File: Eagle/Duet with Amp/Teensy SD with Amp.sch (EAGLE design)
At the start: 20 parts, among them IC2 LM386N-1

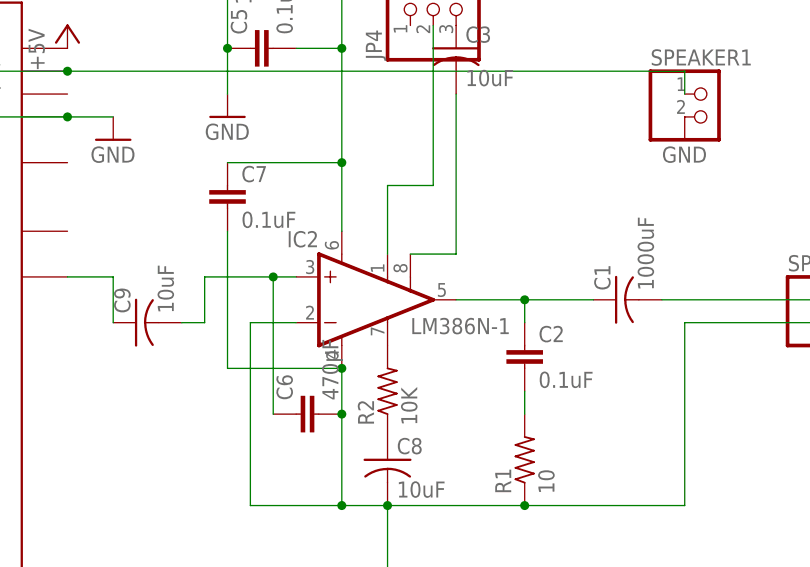
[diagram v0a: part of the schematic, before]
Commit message: Revert "Traced to 32mils"
This reverts commit ffbe95997752b5ed6823b856a1fed8613c21e4f0.
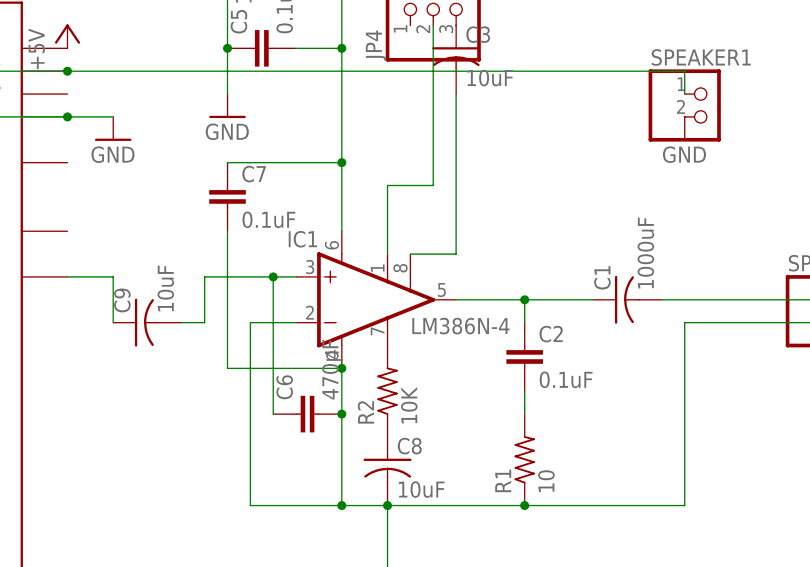
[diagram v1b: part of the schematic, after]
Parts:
- removed IC2: LM386N-1, linear:LM386N-1
- added IC1: LM386N-4, linear:LM386N-4
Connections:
- net +5V: now also IC1.VS; no longer IC2.VS
- net GND: now also IC1.-IN, IC1.GND; no longer IC2.-IN, IC2.GND
- net N$2: now also IC1.GAIN@2; no longer IC2.GAIN@2
- net N$26: now also IC1.GAIN@1; no longer IC2.GAIN@1
- net N$3: now also IC1.OUT; no longer IC2.OUT
- net N$4: now also IC1.BYPASS; no longer IC2.BYPASS
- net N$6: now also IC1.+IN; no longer IC2.+IN
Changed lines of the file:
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@@
 </classes>
 <parts>
+<part name="IC1" library="linear" deviceset="LM386?-*" device="N" technology="4"/>
 <part name="C3" library="rcl" deviceset="C-US" device="025-030X050" value="10uF"/>
 <part name="C8" library="rcl" deviceset="C-US" device="025-030X050" value="10uF"/>
-<part name="C7" library="capacitor-wima" library_urn="urn:adsk.eagle:library:116" deviceset="C" device="2.5/4" value="0.1uF"/>
+<part name="C7" library="capacitor-wima" deviceset="C" device="2.5/4" value="0.1uF"/>
 <part name="R1" library="resistor" deviceset="R-US_" device="0207/7" value="10"/>
 <part name="R2" library="resistor" deviceset="R-US_" device="0207/7" value="10K"/>
-<part name="C2" library="capacitor-wima" library_urn="urn:adsk.eagle:library:116" deviceset="C" device="2.5/4" value="0.1uF"/>
-<part name="C6" library="capacitor-wima" library_urn="urn:adsk.eagle:library:116" deviceset="C" device="2.5/4" value="470pF"/>
+<part name="C2" library="capacitor-wima" deviceset="C" device="2.5/4" value="0.1uF"/>
+<part name="C6" library="capacitor-wima" deviceset="C" device="2.5/4" value="470pF"/>
 <part name="C1" library="rcl" deviceset="C-US" device="025-030X050" value="1000uF"/>
 <part name="SPEAKER" library="pinhead" deviceset="PINHD-1X2" device=""/>
 <part name="C4" library="rcl" deviceset="C-US" device="025-030X050" value="100uF"/>
-<part name="C5" library="capacitor-wima" library_urn="urn:adsk.eagle:library:116" deviceset="C" device="2.5/4" value="0.1uF"/>
-<part name="P+3" library="supply1" library_urn="urn:adsk.eagle:library:371" deviceset="+5V" device=""/>
+<part name="C5" library="capacitor-wima" deviceset="C" device="2.5/4" value="0.1uF"/>
+<part name="P+3" library="supply1" deviceset="+5V" device=""/>
 <part name="U$1" library="Teensy_3_and_LC_Series_Boards_v1.4" deviceset="TEENSY_3.1-3.2_OUTER_ROW" device=""/>
-<part name="GND3" library="supply1" library_urn="urn:adsk.eagle:library:371" deviceset="GND" device=""/>
-<part name="P+1" library="supply1" library_urn="urn:adsk.eagle:library:371" deviceset="+5V" device=""/>
+<part name="GND3" library="supply1" deviceset="GND" device=""/>
+<part name="P+1" library="supply1" deviceset="+5V" device=""/>
 <part name="JP1" library="pinhead" deviceset="PINHD-1X7" device=""/>
 <part name="JP2" library="pinhead" deviceset="PINHD-1X4" device=""/>
-<part name="P+2" library="supply1" library_urn="urn:adsk.eagle:library:371" deviceset="+5V" device=""/>
-<part name="GND4" library="supply1" library_urn="urn:adsk.eagle:library:371" deviceset="GND" device=""/>
+<part name="P+2" library="supply1" deviceset="+5V" device=""/>
+<part name="GND4" library="supply1" deviceset="GND" device=""/>
 <part name="JP3" library="pinhead" deviceset="PINHD-2X9" device=""/>
 <part name="C9" library="rcl" deviceset="C-US" device="025-030X050" value="10uF"/>
 <part name="JP4" library="pinhead" deviceset="PINHD-1X3" device=""/>
-<part name="GND1" library="supply1" library_urn="urn:adsk.eagle:library:371" deviceset="GND" device=""/>
-<part name="GND2" library="supply1" library_urn="urn:adsk.eagle:library:371" deviceset="GND" device=""/>
-<part name="GND5" library="supply1" library_urn="urn:adsk.eagle:library:371" deviceset="GND" device=""/>
+<part name="GND1" library="supply1" deviceset="GND" device=""/>
+<part name="GND2" library="supply1" deviceset="GND" device=""/>
+<part name="GND5" library="supply1" deviceset="GND" device=""/>
 <part name="SPEAKER1" library="pinhead" deviceset="PINHD-1X2" device=""/>
-<part name="GND6" library="supply1" library_urn="urn:adsk.eagle:library:371" deviceset="GND" device=""/>
+<part name="GND6" library="supply1" deviceset="GND" device=""/>
 <part name="SWITCH" library="pinhead" deviceset="PINHD-1X2" device=""/>
-<part name="IC2" library="linear" deviceset="LM386?-*" device="N" technology="1"/>
 </parts>
 <sheets>
@@
 </plain>
 <instances>
+<instance part="IC1" gate="G$1" x="60.96" y="40.64"/>
 <instance part="C3" gate="G$1" x="71.12" y="68.58"/>
 <instance part="C8" gate="G$1" x="63.5" y="22.86"/>
@@
 <instance part="GND6" gate="1" x="96.52" y="58.42"/>
 <instance part="SWITCH" gate="G$1" x="81.28" y="86.36"/>
-<instance part="IC2" gate="G$1" x="60.96" y="40.64"/>
 </instances>
 <busses>
@@
 <pinref part="C3" gate="G$1" pin="2"/>
 <wire x1="71.12" y1="63.5" x2="71.12" y2="45.72" width="0.1524" layer="91"/>
+<pinref part="IC1" gate="G$1" pin="GAIN@2"/>
 <wire x1="71.12" y1="45.72" x2="66.04" y2="45.72" width="0.1524" layer="91"/>
-<pinref part="IC2" gate="G$1" pin="GAIN@2"/>
 </segment>
 </net>
 <net name="N$3" class="0">
 <segment>
+<pinref part="IC1" gate="G$1" pin="OUT"/>
 <wire x1="71.12" y1="40.64" x2="78.74" y2="40.64" width="0.1524" layer="91"/>
 <pinref part="C2" gate="G$1" pin="1"/>
@@
 <junction x="78.74" y="40.64"/>
 <pinref part="C1" gate="G$1" pin="1"/>
-<pinref part="IC2" gate="G$1" pin="OUT"/>
 </segment>
 </net>
@@
 <wire x1="63.5" y1="17.78" x2="58.42" y2="17.78" width="0.1524" layer="91"/>
 <junction x="63.5" y="17.78"/>
+<pinref part="IC1" gate="G$1" pin="GND"/>
 <wire x1="58.42" y1="17.78" x2="58.42" y2="27.94" width="0.1524" layer="91"/>
 <wire x1="58.42" y1="27.94" x2="58.42" y2="33.02" width="0.1524" layer="91"/>
@@
 <wire x1="45.72" y1="48.26" x2="45.72" y2="33.02" width="0.1524" layer="91"/>
 <wire x1="45.72" y1="33.02" x2="58.42" y2="33.02" width="0.1524" layer="91"/>
+<junction x="58.42" y="33.02"/>
 <pinref part="SPEAKER" gate="G$1" pin="2"/>
 <wire x1="111.76" y1="38.1" x2="96.52" y2="38.1" width="0.1524" layer="91"/>
@@
 <wire x1="96.52" y1="17.78" x2="78.74" y2="17.78" width="0.1524" layer="91"/>
 <junction x="78.74" y="17.78"/>
+<pinref part="IC1" gate="G$1" pin="-IN"/>
 <wire x1="53.34" y1="38.1" x2="48.26" y2="38.1" width="0.1524" layer="91"/>
 <wire x1="48.26" y1="38.1" x2="48.26" y2="17.78" width="0.1524" layer="91"/>
 <pinref part="GND1" gate="1" pin="GND"/>
-<pinref part="IC2" gate="G$1" pin="-IN"/>
-<pinref part="IC2" gate="G$1" pin="GND"/>
-<junction x="58.42" y="33.02"/>
 </segment>
 <segment>
@@
 </segment>
 </net>
+<net name="N$4" class="0">
+<segment>
+<pinref part="IC1" gate="G$1" pin="BYPASS"/>
+<pinref part="R2" gate="G$1" pin="2"/>
+</segment>
+</net>
 <net name="N$5" class="0">
 <segment>
@@
 <net name="N$6" class="0">
 <segment>
+<pinref part="IC1" gate="G$1" pin="+IN"/>
 <pinref part="C6" gate="G$1" pin="1"/>
 <wire x1="50.8" y1="43.18" x2="50.8" y2="27.94" width="0.1524" layer="91"/>
@@
 <wire x1="43.18" y1="43.18" x2="50.8" y2="43.18" width="0.1524" layer="91"/>
 <junction x="50.8" y="43.18"/>
-<pinref part="IC2" gate="G$1" pin="+IN"/>
 </segment>
 </net>
 <net name="+5V" class="0">
 <segment>
+<pinref part="IC1" gate="G$1" pin="VS"/>
 <wire x1="58.42" y1="48.26" x2="58.42" y2="55.88" width="0.1524" layer="91"/>
 <pinref part="C7" gate="G$1" pin="1"/>
@@
 <wire x1="78.74" y1="88.9" x2="78.74" y2="86.36" width="0.1524" layer="91"/>
 <junction x="78.74" y="86.36"/>
-<pinref part="IC2" gate="G$1" pin="VS"/>
 </segment>
 <segment>
@@
 <pinref part="JP4" gate="A" pin="2"/>
 <wire x1="68.58" y1="71.12" x2="68.58" y2="53.34" width="0.1524" layer="91"/>
+<pinref part="IC1" gate="G$1" pin="GAIN@1"/>
 <wire x1="68.58" y1="53.34" x2="63.5" y2="53.34" width="0.1524" layer="91"/>
 <wire x1="63.5" y1="53.34" x2="63.5" y2="45.72" width="0.1524" layer="91"/>
-<pinref part="IC2" gate="G$1" pin="GAIN@1"/>
 </segment>
 </net>
@@
 <pinref part="U$1" gate="G$1" pin="2"/>
 <wire x1="-25.4" y1="63.5" x2="-17.78" y2="63.5" width="0.1524" layer="91"/>
-</segment>
-</net>
-<net name="N$4" class="0">
-<segment>
-<pinref part="R2" gate="G$1" pin="2"/>
-<pinref part="IC2" gate="G$1" pin="BYPASS"/>
 </segment>
 </net>
@@
 </schematic>
 </drawing>
-<compatibility>
-<note version="8.2" severity="warning">
-Since Version 8.2, Eagle supports online libraries. The ids
-of those online libraries will not be understood (or retained)
-with this version.
-</note>
-</compatibility>
 </eagle>

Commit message: Traced to 32mils
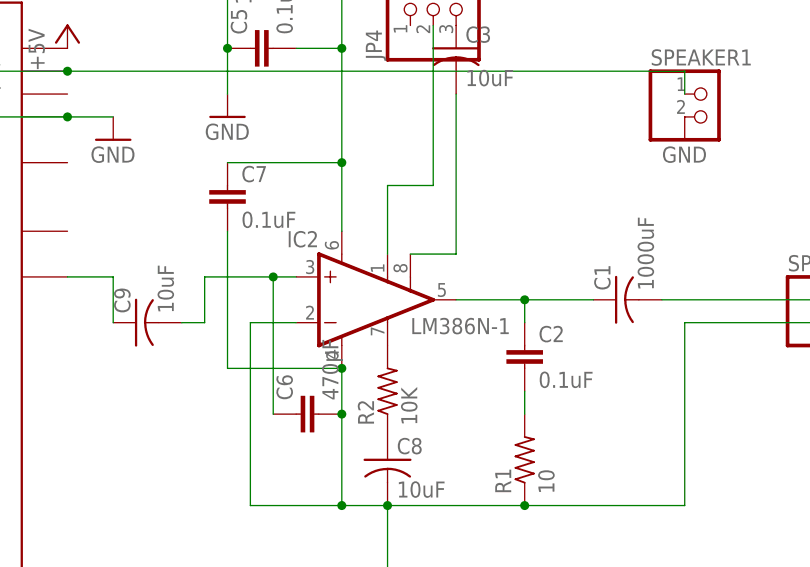
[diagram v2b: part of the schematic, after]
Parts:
- removed IC1: LM386N-4, linear:LM386N-4
- added IC2: LM386N-1, linear:LM386N-1
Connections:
- net +5V: now also IC2.VS; no longer IC1.VS
- net GND: now also IC2.-IN, IC2.GND; no longer IC1.-IN, IC1.GND
- net N$2: now also IC2.GAIN@2; no longer IC1.GAIN@2
- net N$26: now also IC2.GAIN@1; no longer IC1.GAIN@1
- net N$3: now also IC2.OUT; no longer IC1.OUT
- net N$4: now also IC2.BYPASS; no longer IC1.BYPASS
- net N$6: now also IC2.+IN; no longer IC1.+IN
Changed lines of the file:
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@@
 </classes>
 <parts>
-<part name="IC1" library="linear" deviceset="LM386?-*" device="N" technology="4"/>
 <part name="C3" library="rcl" deviceset="C-US" device="025-030X050" value="10uF"/>
 <part name="C8" library="rcl" deviceset="C-US" device="025-030X050" value="10uF"/>
-<part name="C7" library="capacitor-wima" deviceset="C" device="2.5/4" value="0.1uF"/>
+<part name="C7" library="capacitor-wima" library_urn="urn:adsk.eagle:library:116" deviceset="C" device="2.5/4" value="0.1uF"/>
 <part name="R1" library="resistor" deviceset="R-US_" device="0207/7" value="10"/>
 <part name="R2" library="resistor" deviceset="R-US_" device="0207/7" value="10K"/>
-<part name="C2" library="capacitor-wima" deviceset="C" device="2.5/4" value="0.1uF"/>
-<part name="C6" library="capacitor-wima" deviceset="C" device="2.5/4" value="470pF"/>
+<part name="C2" library="capacitor-wima" library_urn="urn:adsk.eagle:library:116" deviceset="C" device="2.5/4" value="0.1uF"/>
+<part name="C6" library="capacitor-wima" library_urn="urn:adsk.eagle:library:116" deviceset="C" device="2.5/4" value="470pF"/>
 <part name="C1" library="rcl" deviceset="C-US" device="025-030X050" value="1000uF"/>
 <part name="SPEAKER" library="pinhead" deviceset="PINHD-1X2" device=""/>
 <part name="C4" library="rcl" deviceset="C-US" device="025-030X050" value="100uF"/>
-<part name="C5" library="capacitor-wima" deviceset="C" device="2.5/4" value="0.1uF"/>
-<part name="P+3" library="supply1" deviceset="+5V" device=""/>
+<part name="C5" library="capacitor-wima" library_urn="urn:adsk.eagle:library:116" deviceset="C" device="2.5/4" value="0.1uF"/>
+<part name="P+3" library="supply1" library_urn="urn:adsk.eagle:library:371" deviceset="+5V" device=""/>
 <part name="U$1" library="Teensy_3_and_LC_Series_Boards_v1.4" deviceset="TEENSY_3.1-3.2_OUTER_ROW" device=""/>
-<part name="GND3" library="supply1" deviceset="GND" device=""/>
-<part name="P+1" library="supply1" deviceset="+5V" device=""/>
+<part name="GND3" library="supply1" library_urn="urn:adsk.eagle:library:371" deviceset="GND" device=""/>
+<part name="P+1" library="supply1" library_urn="urn:adsk.eagle:library:371" deviceset="+5V" device=""/>
 <part name="JP1" library="pinhead" deviceset="PINHD-1X7" device=""/>
 <part name="JP2" library="pinhead" deviceset="PINHD-1X4" device=""/>
-<part name="P+2" library="supply1" deviceset="+5V" device=""/>
-<part name="GND4" library="supply1" deviceset="GND" device=""/>
+<part name="P+2" library="supply1" library_urn="urn:adsk.eagle:library:371" deviceset="+5V" device=""/>
+<part name="GND4" library="supply1" library_urn="urn:adsk.eagle:library:371" deviceset="GND" device=""/>
 <part name="JP3" library="pinhead" deviceset="PINHD-2X9" device=""/>
 <part name="C9" library="rcl" deviceset="C-US" device="025-030X050" value="10uF"/>
 <part name="JP4" library="pinhead" deviceset="PINHD-1X3" device=""/>
-<part name="GND1" library="supply1" deviceset="GND" device=""/>
-<part name="GND2" library="supply1" deviceset="GND" device=""/>
-<part name="GND5" library="supply1" deviceset="GND" device=""/>
+<part name="GND1" library="supply1" library_urn="urn:adsk.eagle:library:371" deviceset="GND" device=""/>
+<part name="GND2" library="supply1" library_urn="urn:adsk.eagle:library:371" deviceset="GND" device=""/>
+<part name="GND5" library="supply1" library_urn="urn:adsk.eagle:library:371" deviceset="GND" device=""/>
 <part name="SPEAKER1" library="pinhead" deviceset="PINHD-1X2" device=""/>
-<part name="GND6" library="supply1" deviceset="GND" device=""/>
+<part name="GND6" library="supply1" library_urn="urn:adsk.eagle:library:371" deviceset="GND" device=""/>
 <part name="SWITCH" library="pinhead" deviceset="PINHD-1X2" device=""/>
+<part name="IC2" library="linear" deviceset="LM386?-*" device="N" technology="1"/>
 </parts>
 <sheets>
@@
 </plain>
 <instances>
-<instance part="IC1" gate="G$1" x="60.96" y="40.64"/>
 <instance part="C3" gate="G$1" x="71.12" y="68.58"/>
 <instance part="C8" gate="G$1" x="63.5" y="22.86"/>
@@
 <instance part="GND6" gate="1" x="96.52" y="58.42"/>
 <instance part="SWITCH" gate="G$1" x="81.28" y="86.36"/>
+<instance part="IC2" gate="G$1" x="60.96" y="40.64"/>
 </instances>
 <busses>
@@
 <pinref part="C3" gate="G$1" pin="2"/>
 <wire x1="71.12" y1="63.5" x2="71.12" y2="45.72" width="0.1524" layer="91"/>
-<pinref part="IC1" gate="G$1" pin="GAIN@2"/>
 <wire x1="71.12" y1="45.72" x2="66.04" y2="45.72" width="0.1524" layer="91"/>
+<pinref part="IC2" gate="G$1" pin="GAIN@2"/>
 </segment>
 </net>
 <net name="N$3" class="0">
 <segment>
-<pinref part="IC1" gate="G$1" pin="OUT"/>
 <wire x1="71.12" y1="40.64" x2="78.74" y2="40.64" width="0.1524" layer="91"/>
 <pinref part="C2" gate="G$1" pin="1"/>
@@
 <junction x="78.74" y="40.64"/>
 <pinref part="C1" gate="G$1" pin="1"/>
+<pinref part="IC2" gate="G$1" pin="OUT"/>
 </segment>
 </net>
@@
 <wire x1="63.5" y1="17.78" x2="58.42" y2="17.78" width="0.1524" layer="91"/>
 <junction x="63.5" y="17.78"/>
-<pinref part="IC1" gate="G$1" pin="GND"/>
 <wire x1="58.42" y1="17.78" x2="58.42" y2="27.94" width="0.1524" layer="91"/>
 <wire x1="58.42" y1="27.94" x2="58.42" y2="33.02" width="0.1524" layer="91"/>
@@
 <wire x1="45.72" y1="48.26" x2="45.72" y2="33.02" width="0.1524" layer="91"/>
 <wire x1="45.72" y1="33.02" x2="58.42" y2="33.02" width="0.1524" layer="91"/>
-<junction x="58.42" y="33.02"/>
 <pinref part="SPEAKER" gate="G$1" pin="2"/>
 <wire x1="111.76" y1="38.1" x2="96.52" y2="38.1" width="0.1524" layer="91"/>
@@
 <wire x1="96.52" y1="17.78" x2="78.74" y2="17.78" width="0.1524" layer="91"/>
 <junction x="78.74" y="17.78"/>
-<pinref part="IC1" gate="G$1" pin="-IN"/>
 <wire x1="53.34" y1="38.1" x2="48.26" y2="38.1" width="0.1524" layer="91"/>
 <wire x1="48.26" y1="38.1" x2="48.26" y2="17.78" width="0.1524" layer="91"/>
 <pinref part="GND1" gate="1" pin="GND"/>
+<pinref part="IC2" gate="G$1" pin="-IN"/>
+<pinref part="IC2" gate="G$1" pin="GND"/>
+<junction x="58.42" y="33.02"/>
 </segment>
 <segment>
@@
 </segment>
 </net>
-<net name="N$4" class="0">
-<segment>
-<pinref part="IC1" gate="G$1" pin="BYPASS"/>
-<pinref part="R2" gate="G$1" pin="2"/>
-</segment>
-</net>
 <net name="N$5" class="0">
 <segment>
@@
 <net name="N$6" class="0">
 <segment>
-<pinref part="IC1" gate="G$1" pin="+IN"/>
 <pinref part="C6" gate="G$1" pin="1"/>
 <wire x1="50.8" y1="43.18" x2="50.8" y2="27.94" width="0.1524" layer="91"/>
@@
 <wire x1="43.18" y1="43.18" x2="50.8" y2="43.18" width="0.1524" layer="91"/>
 <junction x="50.8" y="43.18"/>
+<pinref part="IC2" gate="G$1" pin="+IN"/>
 </segment>
 </net>
 <net name="+5V" class="0">
 <segment>
-<pinref part="IC1" gate="G$1" pin="VS"/>
 <wire x1="58.42" y1="48.26" x2="58.42" y2="55.88" width="0.1524" layer="91"/>
 <pinref part="C7" gate="G$1" pin="1"/>
@@
 <wire x1="78.74" y1="88.9" x2="78.74" y2="86.36" width="0.1524" layer="91"/>
 <junction x="78.74" y="86.36"/>
+<pinref part="IC2" gate="G$1" pin="VS"/>
 </segment>
 <segment>
@@
 <pinref part="JP4" gate="A" pin="2"/>
 <wire x1="68.58" y1="71.12" x2="68.58" y2="53.34" width="0.1524" layer="91"/>
-<pinref part="IC1" gate="G$1" pin="GAIN@1"/>
 <wire x1="68.58" y1="53.34" x2="63.5" y2="53.34" width="0.1524" layer="91"/>
 <wire x1="63.5" y1="53.34" x2="63.5" y2="45.72" width="0.1524" layer="91"/>
+<pinref part="IC2" gate="G$1" pin="GAIN@1"/>
 </segment>
 </net>
@@
 <pinref part="U$1" gate="G$1" pin="2"/>
 <wire x1="-25.4" y1="63.5" x2="-17.78" y2="63.5" width="0.1524" layer="91"/>
+</segment>
+</net>
+<net name="N$4" class="0">
+<segment>
+<pinref part="R2" gate="G$1" pin="2"/>
+<pinref part="IC2" gate="G$1" pin="BYPASS"/>
 </segment>
 </net>
@@
 </schematic>
 </drawing>
+<compatibility>
+<note version="8.2" severity="warning">
+Since Version 8.2, Eagle supports online libraries. The ids
+of those online libraries will not be understood (or retained)
+with this version.
+</note>
+</compatibility>
 </eagle>
